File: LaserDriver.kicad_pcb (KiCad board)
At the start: 2 copper layers, 26 parts, among them J100 Screw_Terminal_01x04, J102 Screw_Terminal_01x02, U1 TPS92513DGQR

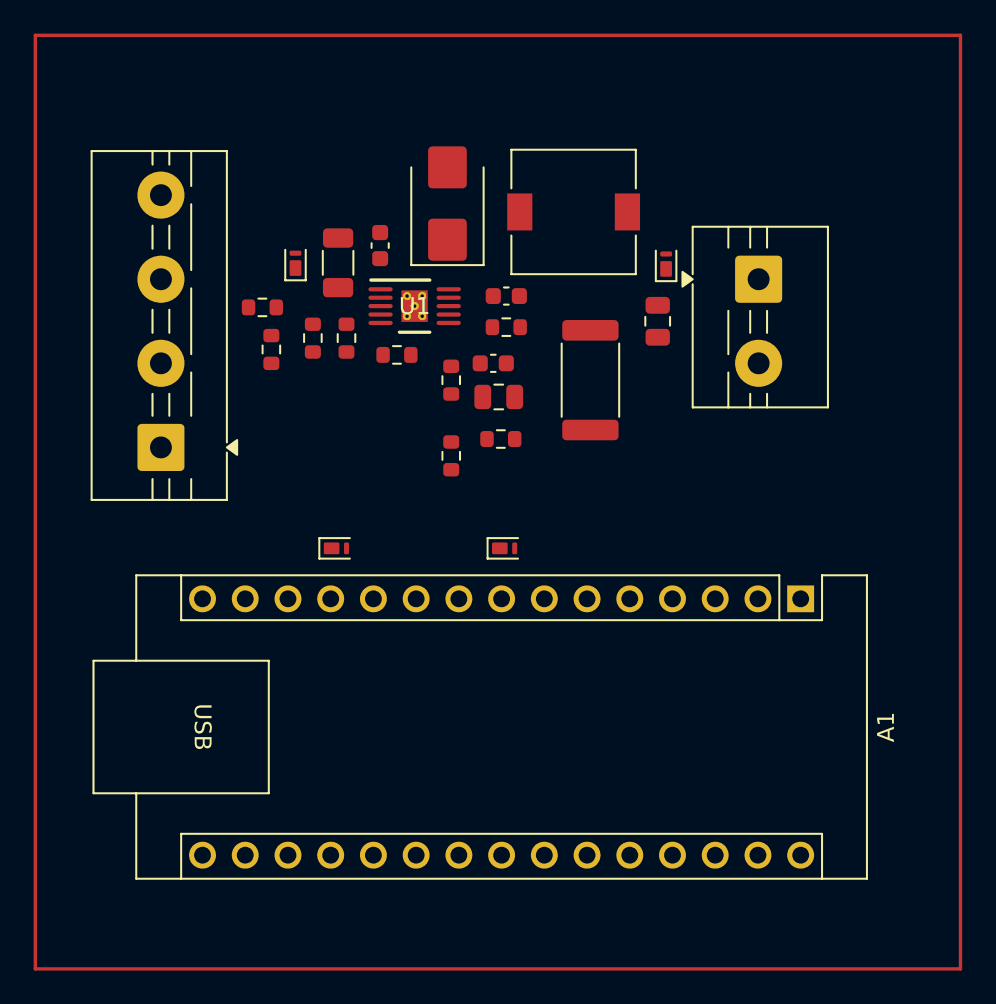
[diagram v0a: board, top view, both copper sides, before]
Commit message: finihsed placing
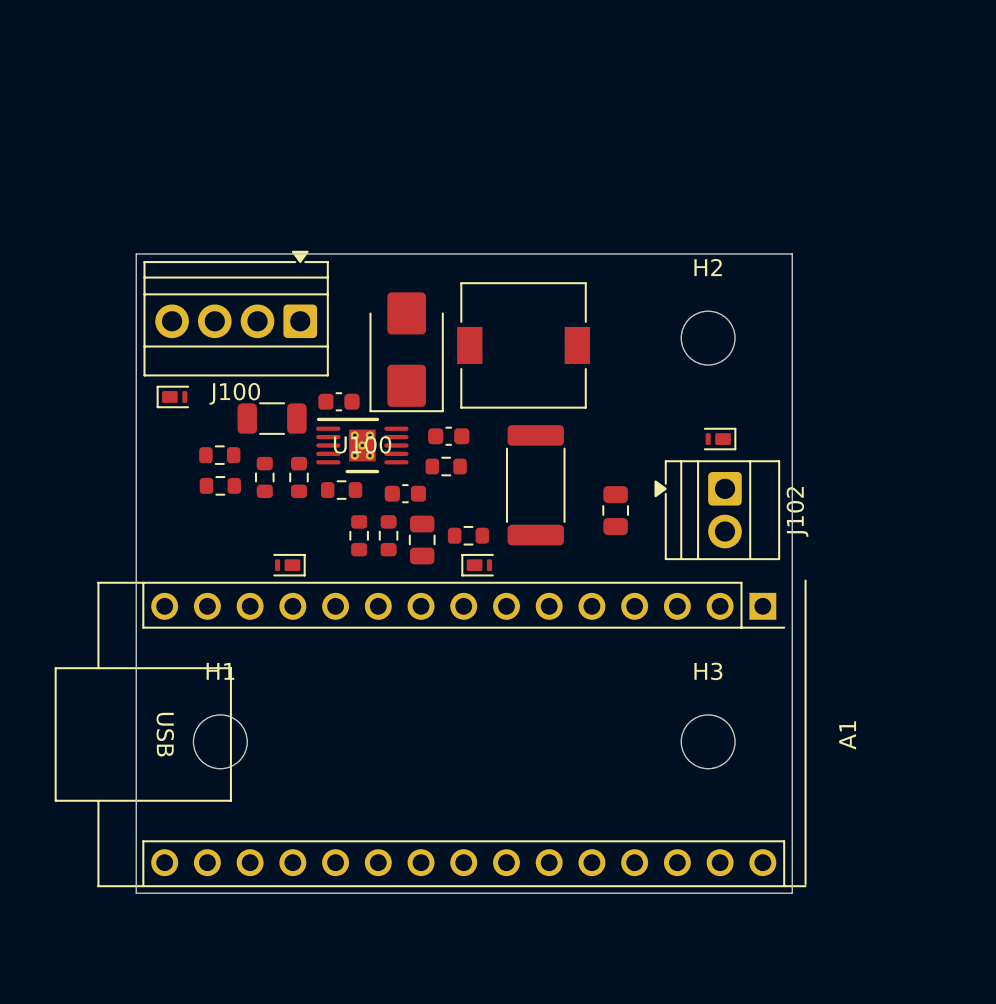
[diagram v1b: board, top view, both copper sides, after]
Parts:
- added H1: MountingHole, MountingHole:MountingHole_3.2mm_M3, F.Cu at (35.0, 128.0)
- added H2: MountingHole, MountingHole:MountingHole_3.2mm_M3, F.Cu at (64.0, 104.0)
- added H3: MountingHole, MountingHole:MountingHole_3.2mm_M3, F.Cu at (64.0, 128.0)
- J100: footprint TerminalBlock:TerminalBlock_MaiXu_MX126-5.0-04P_1x04_P5.00mm -> TerminalBlock:TerminalBlock_Xinya_XY308-2.54-4P_1x04_P2.54mm_Horizontal
- J102: footprint TerminalBlock:TerminalBlock_MaiXu_MX126-5.0-02P_1x02_P5.00mm -> TerminalBlock:TerminalBlock_Xinya_XY308-2.54-2P_1x02_P2.54mm_Horizontal
- moved J102 12.6 mm to (65.0, 113.0)
- moved C104 11.5 mm to (58.5, 114.2)
- moved J100 11.2 mm to (39.8, 103.0), turned to 180 degrees
- moved D102 10.9 mm to (64.6, 110.0), turned to 180 degrees
- moved D100 10.7 mm to (32.3, 107.5), turned to 0 degrees
- moved R108 10.2 mm to (43.2, 115.8), turned to 90 degrees
- moved C100 10.1 mm to (38.1, 108.8), turned to 180 degrees
- moved R106 9.97 mm to (45.0, 115.8)
- moved C106 9.64 mm to (47.0, 116.0), turned to 90 degrees
- moved C103 9.60 mm to (42.0, 107.8), turned to 0 degrees
- moved C105 9.35 mm to (46.0, 113.2)
- moved R111 9.14 mm to (35.0, 111.0)
- moved R104 9.02 mm to (48.4, 111.6)
- moved D101 9.02 mm to (46.1, 104.7)
- moved C102 9.01 mm to (48.6, 109.8)
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- renumbered U1 to U100
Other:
- board outline added: 39 x 38 mm
